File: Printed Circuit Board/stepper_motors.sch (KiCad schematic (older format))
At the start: 10 parts, among them J11 Conn_02x03_Odd_Even, J7 Conn_01x04_Male, J8 Conn_01x04_Male, J9 Conn_02x03_Odd_Even

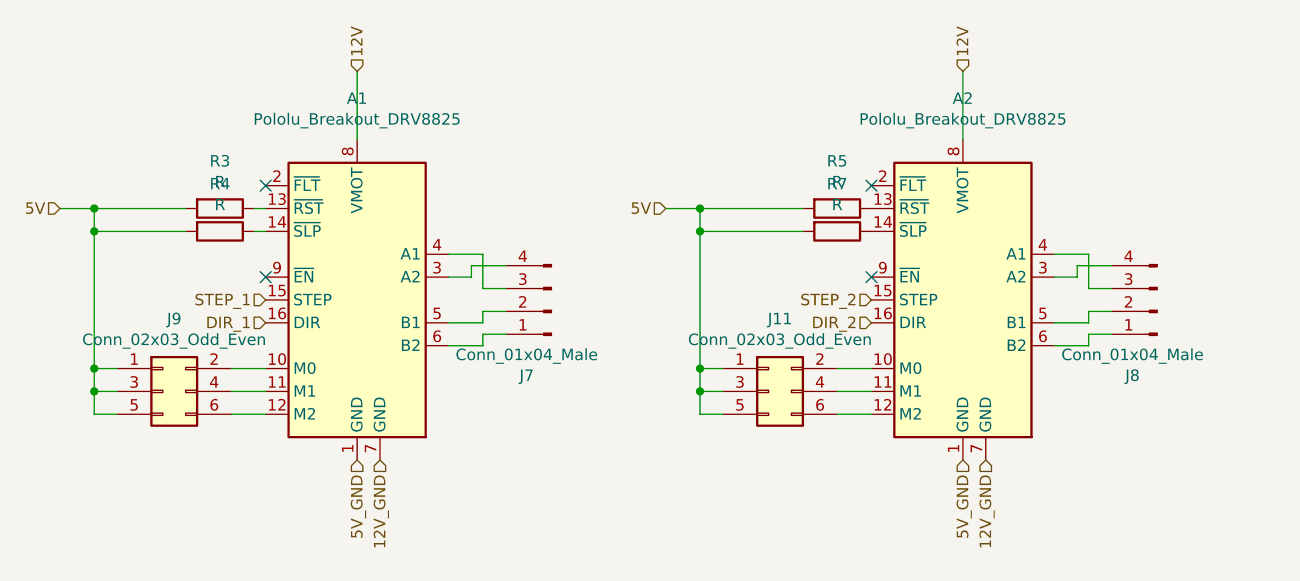
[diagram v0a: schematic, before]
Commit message: PCB physical board
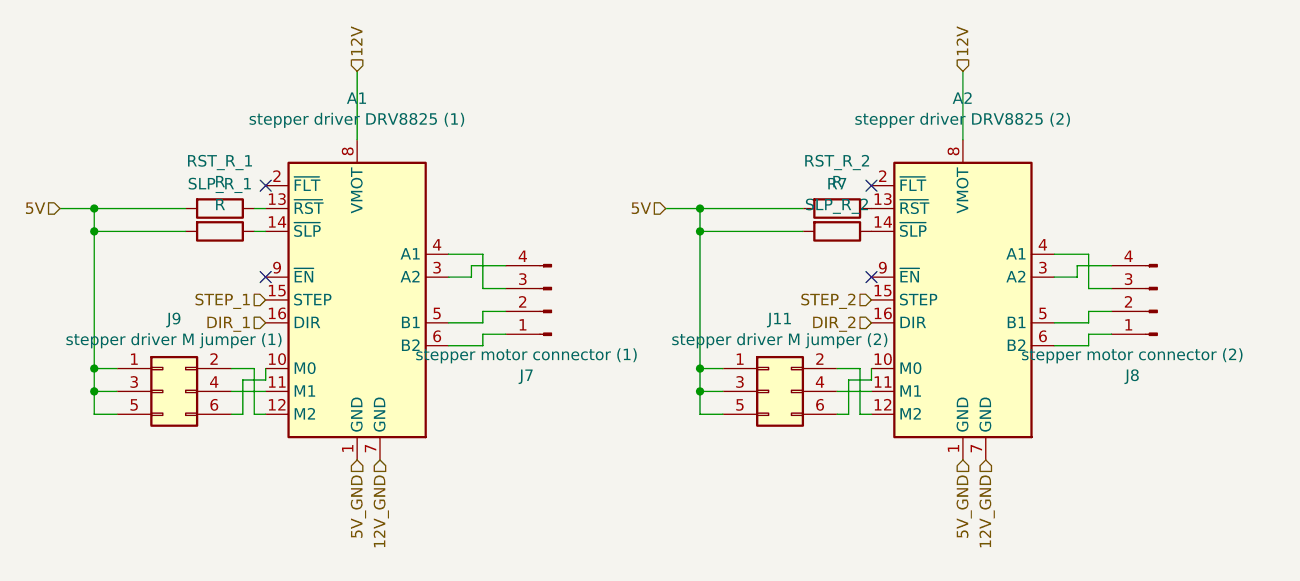
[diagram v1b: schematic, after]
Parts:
- A1: value Pololu_Breakout_DRV8825 -> stepper driver DRV8825 (1)
- A2: value Pololu_Breakout_DRV8825 -> stepper driver DRV8825 (2)
- J11: value Conn_02x03_Odd_Even -> stepper driver M jumper (2)
- J7: value Conn_01x04_Male -> stepper motor connector (1)
- J8: value Conn_01x04_Male -> stepper motor connector (2)
- J9: value Conn_02x03_Odd_Even -> stepper driver M jumper (1); footprint Connector_PinSocket_2.54mm:PinSocket_2x03_P2.54mm_Horizontal -> Connector_PinSocket_2.54mm:PinSocket_2x03_P2.54mm_Vertical
- R7: value R -> SLP_R_2
- renumbered R3 to RST_R_1, R5 to RST_R_2, R4 to SLP_R_1
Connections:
- net at J11.2 (Pin_2): now also A2.12 (M2); no longer A2.10 (M0)
- net at J11.6 (Pin_6): now also A2.10 (M0); no longer A2.12 (M2)
- net at J9.2 (Pin_2): now also A1.12 (M2); no longer A1.10 (M0)
- net at J9.6 (Pin_6): now also A1.10 (M0); no longer A1.12 (M2)
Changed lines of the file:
@@
 AR Path="/603B418F/603C2499" Ref="J8"  Part="1"
 F 0 "J8" H 8308 4681 50  0000 C CNN
-F 1 "Conn_01x04_Male" H 8308 4590 50  0000 C CNN
+F 1 "stepper motor connector (2)" H 8308 4590 50  0000 C CNN
 F 2 "Connector_PinHeader_2.54mm:PinHeader_1x04_P2.54mm_Vertical" H 8200 4400 50  0001 C CNN
 F 3 "~" H 8200 4400 50  0001 C CNN
@@
 AR Path="/603B418F/603C24AC" Ref="J7"  Part="1"
 F 0 "J7" H 5658 4681 50  0000 C CNN
-F 1 "Conn_01x04_Male" H 5658 4590 50  0000 C CNN
+F 1 "stepper motor connector (1)" H 5658 4590 50  0000 C CNN
 F 2 "Connector_PinHeader_2.54mm:PinHeader_1x04_P2.54mm_Vertical" H 5550 4400 50  0001 C CNN
 F 3 "~" H 5550 4400 50  0001 C CNN
@@
 AR Path="/603B418F/603C24C6" Ref="A2"  Part="1"
 F 0 "A2" H 7350 5031 50  0000 C CNN
-F 1 "Pololu_Breakout_DRV8825" H 7350 4940 50  0000 C CNN
+F 1 "stepper driver DRV8825 (2)" H 7350 4940 50  0000 C CNN
 F 2 "Module:Pololu_Breakout-16_15.2x20.3mm" H 7550 3450 50  0001 L CNN
 F 3 "https://www.pololu.com/product/2982" H 7450 3950 50  0001 C CNN
@@
 P 6800 3950
 AR Path="/603C24CC" Ref="R?"  Part="1"
-AR Path="/603B418F/603C24CC" Ref="R5"  Part="1"
-F 0 "R5" V 6593 3950 50  0000 C CNN
+AR Path="/603B418F/603C24CC" Ref="RST_R_2"  Part="1"
+F 0 "RST_R_2" V 6593 3950 50  0000 C CNN
 F 1 "R" V 6684 3950 50  0000 C CNN
 F 2 "Resistor_SMD:R_1206_3216Metric" V 6730 3950 50  0001 C CNN
@@
 AR Path="/603B418F/603C24D3" Ref="R7"  Part="1"
 F 0 "R7" V 6593 4050 50  0000 C CNN
-F 1 "R" V 6684 4050 50  0000 C CNN
+F 1 "SLP_R_2" V 6684 4050 50  0000 C CNN
 F 2 "Resistor_SMD:R_1206_3216Metric" V 6730 4050 50  0001 C CNN
 F 3 "~" H 6800 4050 50  0001 C CNN
@@
 P 4100 4050
 AR Path="/603D354E" Ref="R?"  Part="1"
-AR Path="/603B418F/603D354E" Ref="R4"  Part="1"
-F 0 "R4" V 3893 4050 50  0000 C CNN
+AR Path="/603B418F/603D354E" Ref="SLP_R_1"  Part="1"
+F 0 "SLP_R_1" V 3893 4050 50  0000 C CNN
 F 1 "R" V 3984 4050 50  0000 C CNN
 F 2 "Resistor_SMD:R_1206_3216Metric" V 4030 4050 50  0001 C CNN
@@
 P 4100 3950
 AR Path="/603D41C9" Ref="R?"  Part="1"
-AR Path="/603B418F/603D41C9" Ref="R3"  Part="1"
-F 0 "R3" V 3893 3950 50  0000 C CNN
+AR Path="/603B418F/603D41C9" Ref="RST_R_1"  Part="1"
+F 0 "RST_R_1" V 3893 3950 50  0000 C CNN
 F 1 "R" V 3984 3950 50  0000 C CNN
 F 2 "Resistor_SMD:R_1206_3216Metric" V 4030 3950 50  0001 C CNN
@@
 P 6500 4750
 F 0 "J11" H 6550 5067 50  0000 C CNN
-F 1 "Conn_02x03_Odd_Even" H 6550 4976 50  0000 C CNN
+F 1 "stepper driver M jumper (2)" H 6550 4976 50  0000 C CNN
 F 2 "Connector_PinSocket_2.54mm:PinSocket_2x03_P2.54mm_Vertical" H 6500 4750 50  0001 C CNN
 F 3 "~" H 6500 4750 50  0001 C CNN
@@
 $EndComp
 Wire Wire Line
-	6800 4650 6950 4650
-Wire Wire Line
 	6800 4750 6950 4750
-Wire Wire Line
-	6950 4850 6800 4850
 Wire Wire Line
 	6300 4650 6200 4650
@@
 P 3850 4750
 F 0 "J9" H 3900 5067 50  0000 C CNN
-F 1 "Conn_02x03_Odd_Even" H 3900 4976 50  0000 C CNN
-F 2 "Connector_PinSocket_2.54mm:PinSocket_2x03_P2.54mm_Horizontal" H 3850 4750 50  0001 C CNN
+F 1 "stepper driver M jumper (1)" H 3900 4976 50  0000 C CNN
+F 2 "Connector_PinSocket_2.54mm:PinSocket_2x03_P2.54mm_Vertical" H 3850 4750 50  0001 C CNN
 F 3 "~" H 3850 4750 50  0001 C CNN
 	1    3850 4750
@@
 $EndComp
 Wire Wire Line
-	4150 4650 4300 4650
-Wire Wire Line
 	4150 4750 4300 4750
-Wire Wire Line
-	4300 4850 4150 4850
 Wire Wire Line
 	3650 4650 3550 4650
@@
 AR Path="/603B418F/603C24B3" Ref="A1"  Part="1"
 F 0 "A1" H 4700 5031 50  0000 C CNN
-F 1 "Pololu_Breakout_DRV8825" H 4700 4940 50  0000 C CNN
+F 1 "stepper driver DRV8825 (1)" H 4700 4940 50  0000 C CNN
 F 2 "Module:Pololu_Breakout-16_15.2x20.3mm" H 4900 3450 50  0001 L CNN
 F 3 "https://www.pololu.com/product/2982" H 4800 3950 50  0001 C CNN
@@
 Wire Wire Line
 	3550 4050 3550 4650
+Wire Wire Line
+	4150 4650 4250 4650
+Wire Wire Line
+	4250 4650 4250 4850
+Wire Wire Line
+	4250 4850 4300 4850
+Wire Wire Line
+	4300 4650 4300 4700
+Wire Wire Line
+	4300 4700 4200 4700
+Wire Wire Line
+	4200 4700 4200 4850
+Wire Wire Line
+	4200 4850 4150 4850
+Wire Wire Line
+	6800 4650 6900 4650
+Wire Wire Line
+	6900 4650 6900 4850
+Wire Wire Line
+	6900 4850 6950 4850
+Wire Wire Line
+	6950 4650 6950 4700
+Wire Wire Line
+	6950 4700 6850 4700
+Wire Wire Line
+	6850 4700 6850 4850
+Wire Wire Line
+	6850 4850 6800 4850
 $EndSCHEMATC
